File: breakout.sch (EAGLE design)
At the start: 11 parts, among them IC2 REG1117

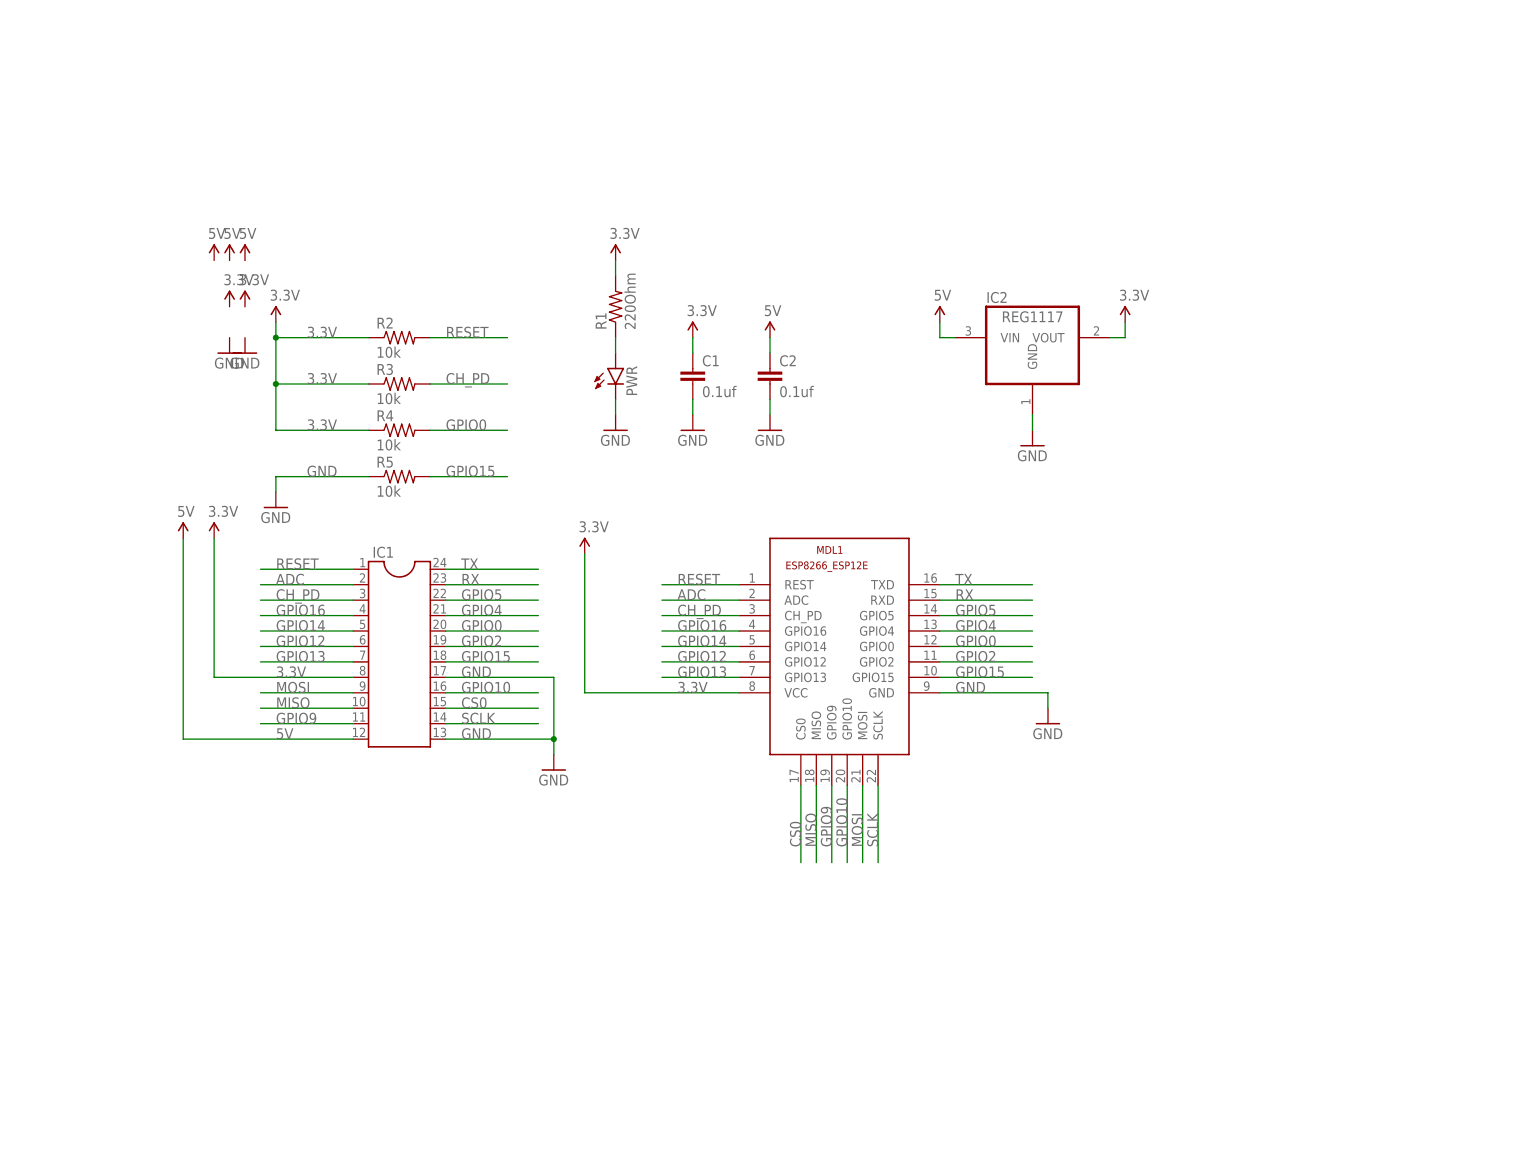
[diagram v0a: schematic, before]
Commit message: Tidy up for publishing
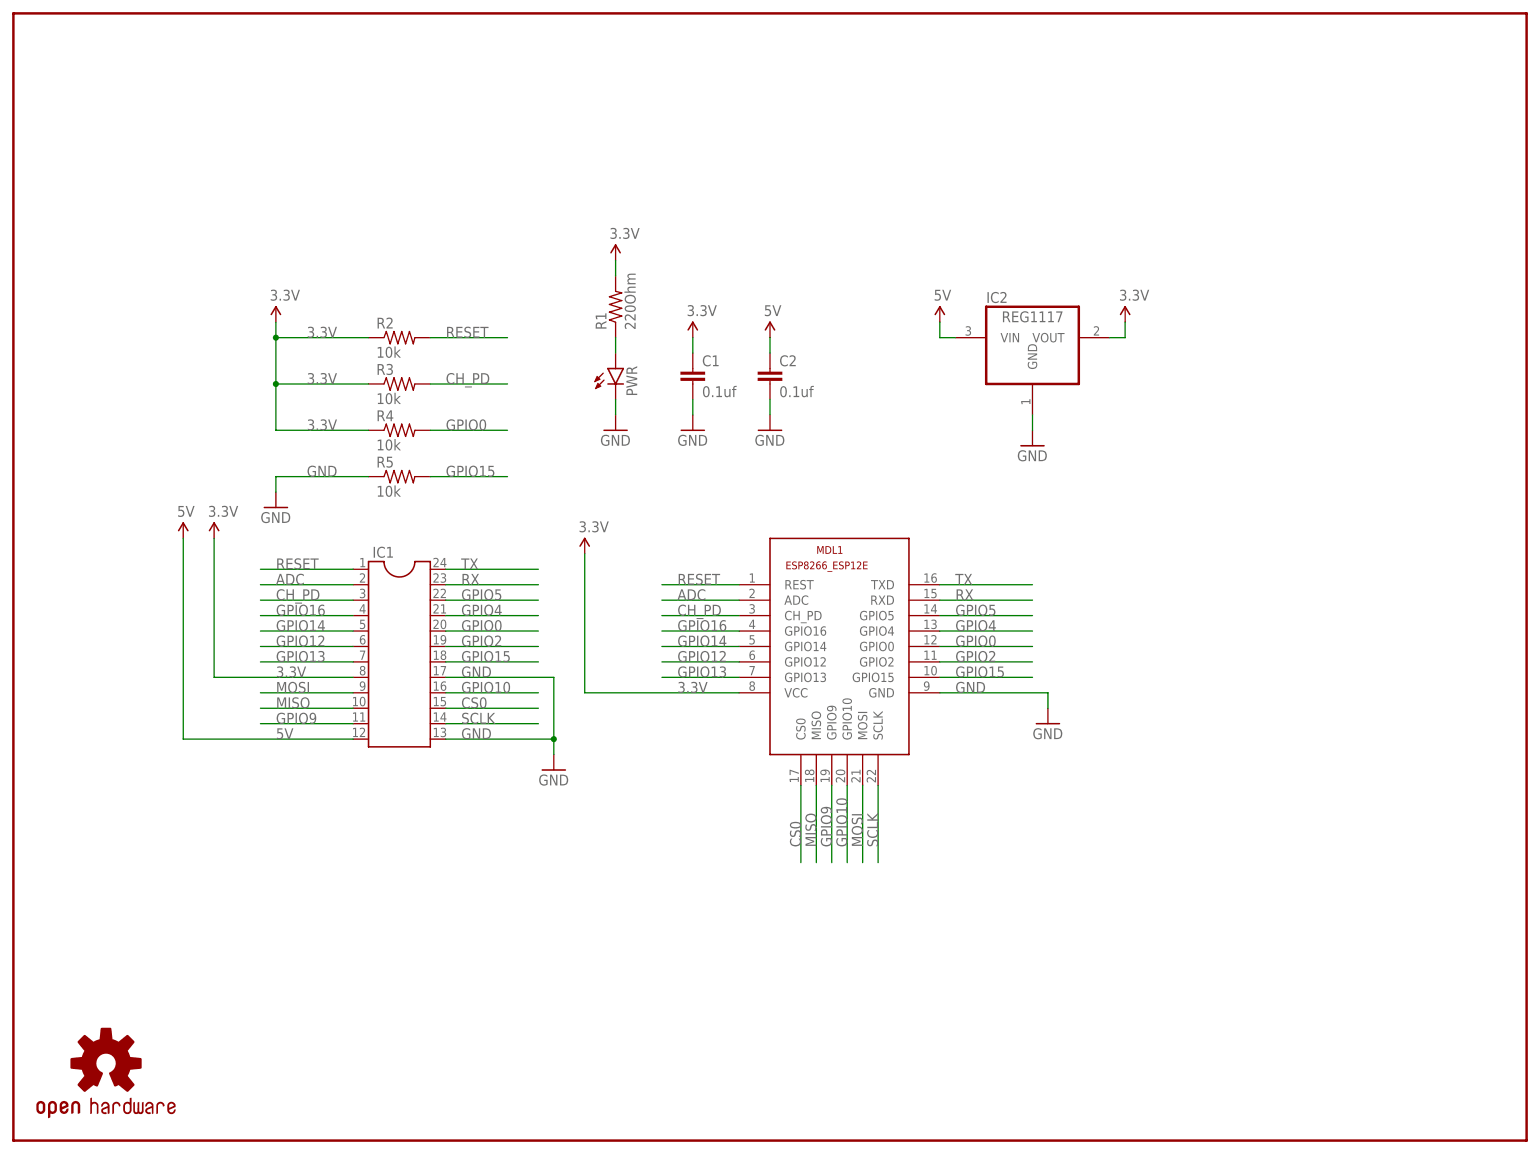
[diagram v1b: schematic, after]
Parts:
- added FRAME1: (no value), SparkFun-Aesthetics:FRAME-LETTERNO_PACKAGE
- added LOGO1: OSHW-LOGOS, SparkFun-Aesthetics:OSHW-LOGOS
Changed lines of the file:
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@@
 <layer number="112" name="tSilk" color="7" fill="1" visible="yes" active="yes"/>
 <layer number="113" name="IDFDebug" color="4" fill="1" visible="yes" active="yes"/>
+<layer number="114" name="FRNTMAAT1" color="7" fill="1" visible="yes" active="yes"/>
+<layer number="115" name="FRNTMAAT2" color="7" fill="1" visible="yes" active="yes"/>
 <layer number="116" name="Patch_BOT" color="9" fill="4" visible="no" active="yes"/>
+<layer number="117" name="BACKMAAT1" color="7" fill="1" visible="yes" active="yes"/>
+<layer number="118" name="Rect_Pads" color="7" fill="1" visible="no" active="no"/>
+<layer number="119" name="KAP_TEKEN" color="7" fill="1" visible="yes" active="yes"/>
+<layer number="120" name="KAP_MAAT1" color="7" fill="1" visible="yes" active="yes"/>
 <layer number="121" name="_tsilk" color="7" fill="1" visible="no" active="yes"/>
 <layer number="122" name="_bsilk" color="7" fill="1" visible="no" active="yes"/>
@@
 <layer number="128" name="_bValues" color="7" fill="1" visible="yes" active="yes"/>
 <layer number="129" name="Mask" color="7" fill="1" visible="yes" active="yes"/>
+<layer number="130" name="SMDSTROOK" color="7" fill="1" visible="yes" active="yes"/>
 <layer number="131" name="tAdjust" color="7" fill="1" visible="yes" active="yes"/>
 <layer number="132" name="bAdjust" color="7" fill="1" visible="yes" active="yes"/>
@@
 <layer number="230" name="230bmp" color="7" fill="1" visible="yes" active="yes"/>
 <layer number="231" name="231bmp" color="7" fill="1" visible="yes" active="yes"/>
+<layer number="232" name="Eagle3D_PG2" color="7" fill="1" visible="no" active="no"/>
+<layer number="233" name="Eagle3D_PG3" color="7" fill="1" visible="no" active="no"/>
 <layer number="248" name="Housing" color="7" fill="1" visible="yes" active="yes"/>
 <layer number="249" name="Edge" color="7" fill="1" visible="yes" active="yes"/>
@@
 <part name="C1" library="SparkFun-Capacitors" deviceset="CAP" device="1206" value="0.1uf"/>
 <part name="C2" library="SparkFun-Capacitors" deviceset="CAP" device="1206" value="0.1uf"/>
-<part name="GND1" library="supply1" deviceset="GND" device=""/>
 <part name="GND2" library="supply1" deviceset="GND" device=""/>
 <part name="GND3" library="supply1" deviceset="GND" device=""/>
@@
 <part name="GND7" library="supply1" deviceset="GND" device=""/>
 <part name="GND8" library="supply1" deviceset="GND" device=""/>
-<part name="GND9" library="supply1" deviceset="GND" device=""/>
 <part name="IC2" library="burr-brown" deviceset="REG1117" device=""/>
 <part name="SUPPLY1" library="SparkFun-Aesthetics" deviceset="3.3V" device=""/>
-<part name="SUPPLY2" library="SparkFun-Aesthetics" deviceset="3.3V" device=""/>
 <part name="SUPPLY3" library="SparkFun-Aesthetics" deviceset="3.3V" device=""/>
 <part name="SUPPLY4" library="SparkFun-Aesthetics" deviceset="3.3V" device=""/>
 <part name="SUPPLY5" library="SparkFun-Aesthetics" deviceset="3.3V" device=""/>
 <part name="SUPPLY6" library="SparkFun-Aesthetics" deviceset="3.3V" device=""/>
-<part name="SUPPLY7" library="SparkFun-Aesthetics" deviceset="3.3V" device=""/>
 <part name="SUPPLY8" library="SparkFun-Aesthetics" deviceset="3.3V" device=""/>
-<part name="SUPPLY9" library="SparkFun-Aesthetics" deviceset="5V" device=""/>
-<part name="SUPPLY10" library="SparkFun-Aesthetics" deviceset="5V" device=""/>
-<part name="SUPPLY11" library="SparkFun-Aesthetics" deviceset="5V" device=""/>
 <part name="SUPPLY12" library="SparkFun-Aesthetics" deviceset="5V" device=""/>
 <part name="SUPPLY13" library="SparkFun-Aesthetics" deviceset="5V" device=""/>
@@
 <part name="R4" library="SparkFun-Resistors" deviceset="RESISTOR" device="1206" value="10k"/>
 <part name="R5" library="SparkFun-Resistors" deviceset="RESISTOR" device="1206" value="10k"/>
+<part name="LOGO1" library="SparkFun-Aesthetics" deviceset="OSHW-LOGO" device="S"/>
+<part name="FRAME1" library="SparkFun-Aesthetics" deviceset="FRAME-LETTER" device="NO_PACKAGE"/>
 </parts>
 <sheets>
@@
 <instance part="C1" gate="G$1" x="66.04" y="83.82"/>
 <instance part="C2" gate="G$1" x="78.74" y="83.82"/>
-<instance part="GND1" gate="1" x="-10.16" y="88.9"/>
 <instance part="GND2" gate="1" x="53.34" y="76.2"/>
 <instance part="GND3" gate="1" x="43.18" y="20.32"/>
@@
 <instance part="GND7" gate="1" x="121.92" y="73.66"/>
 <instance part="GND8" gate="1" x="-2.54" y="63.5"/>
-<instance part="GND9" gate="1" x="-7.62" y="88.9"/>
 <instance part="IC2" gate="G$1" x="121.92" y="91.44"/>
 <instance part="SUPPLY1" gate="G$1" x="53.34" y="104.14"/>
-<instance part="SUPPLY2" gate="G$1" x="-7.62" y="96.52"/>
 <instance part="SUPPLY3" gate="G$1" x="137.16" y="93.98"/>
 <instance part="SUPPLY4" gate="G$1" x="-12.7" y="58.42"/>
 <instance part="SUPPLY5" gate="G$1" x="66.04" y="91.44"/>
 <instance part="SUPPLY6" gate="G$1" x="48.26" y="55.88"/>
-<instance part="SUPPLY7" gate="G$1" x="-10.16" y="96.52"/>
 <instance part="SUPPLY8" gate="G$1" x="-2.54" y="93.98"/>
-<instance part="SUPPLY9" gate="G$1" x="-12.7" y="104.14"/>
-<instance part="SUPPLY10" gate="G$1" x="-10.16" y="104.14"/>
-<instance part="SUPPLY11" gate="G$1" x="-7.62" y="104.14"/>
 <instance part="SUPPLY12" gate="G$1" x="-17.78" y="58.42"/>
 <instance part="SUPPLY13" gate="G$1" x="78.74" y="91.44"/>
@@
 <instance part="R4" gate="G$1" x="17.78" y="76.2"/>
 <instance part="R5" gate="G$1" x="17.78" y="68.58"/>
+<instance part="LOGO1" gate="G$1" x="-30.48" y="-27.94"/>
+<instance part="FRAME1" gate="G$1" x="-45.72" y="-40.64"/>
 </instances>
 <busses>
